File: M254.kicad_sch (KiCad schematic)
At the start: 14 parts, among them J1 from Sensor, J2 to M304, U1 NJM2903

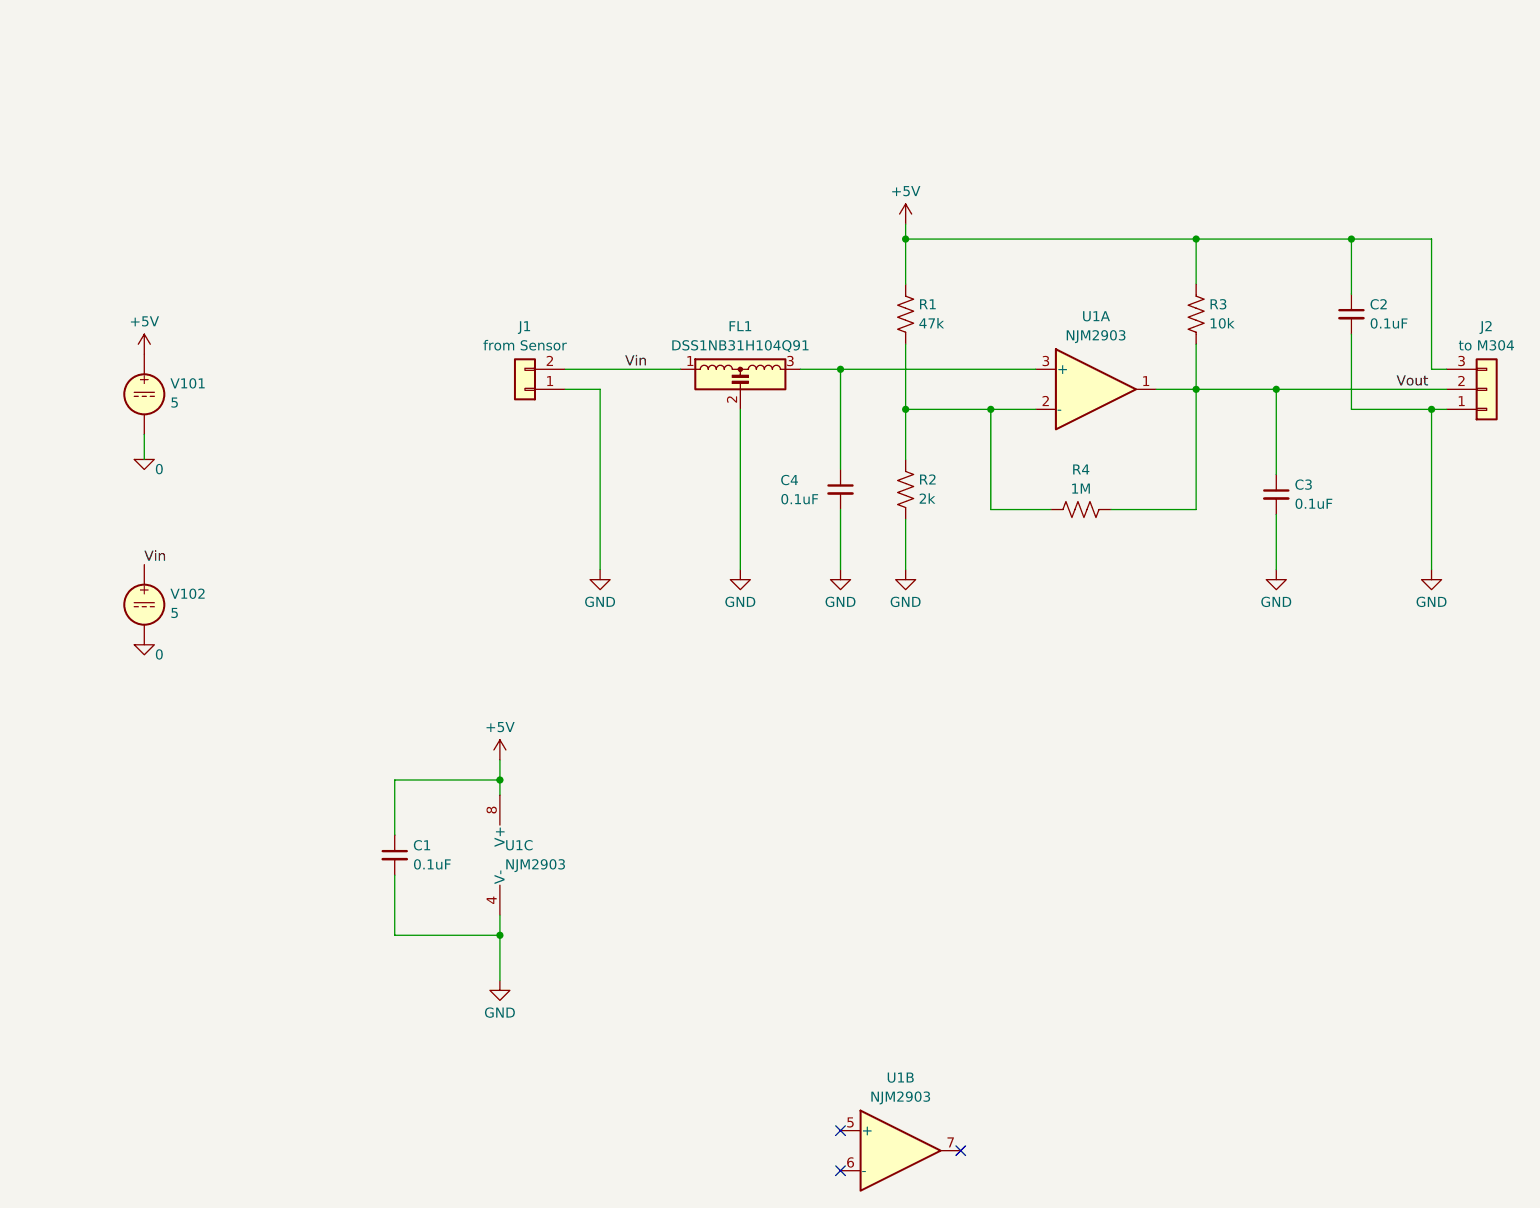
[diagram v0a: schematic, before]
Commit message: 途中
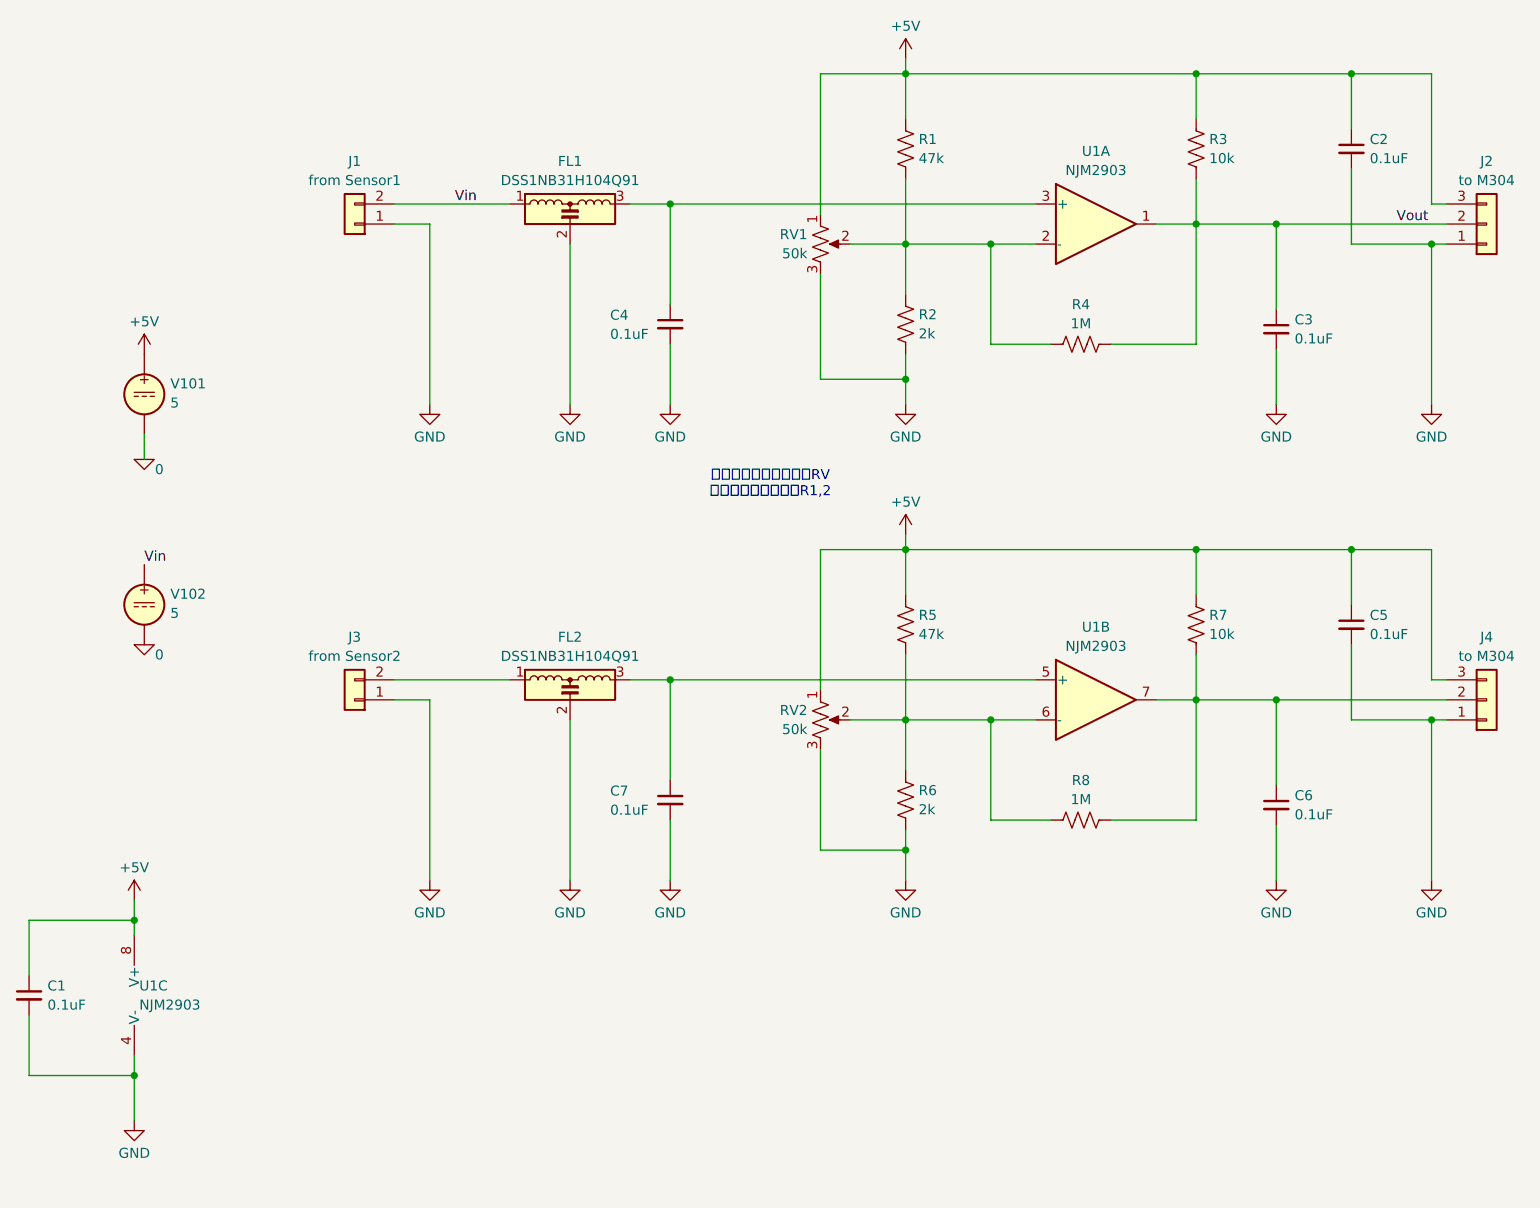
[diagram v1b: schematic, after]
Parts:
- added C5, C6, C7: 0.1uF, Capacitor_THT:C_Disc_D3.4mm_W2.1mm_P2.50mm, symbol Device:C_Small
- added FL2: DSS1NB31H104Q91, HOLLY2:DSS1, symbol Device:Filter_EMI_LCL
- added J3: from Sensor2, Connector_JST:JST_XH_B2B-XH-A_1x02_P2.50mm_Vertical, symbol Connector_Generic:Conn_01x02
- added J4: to M304, Connector_JST:JST_XH_B3B-XH-A_1x03_P2.50mm_Vertical, symbol Connector_Generic:Conn_01x03
- added R5: 47k, Resistor_THT:R_Axial_DIN0207_L6.3mm_D2.5mm_P2.54mm_Vertical, symbol Device:R_US
- added R6: 2k, Resistor_THT:R_Axial_DIN0207_L6.3mm_D2.5mm_P2.54mm_Vertical, symbol Device:R_US
- added R7: 10k, Resistor_THT:R_Axial_DIN0207_L6.3mm_D2.5mm_P2.54mm_Vertical, symbol Device:R_US
- added R8: 1M, Resistor_THT:R_Axial_DIN0207_L6.3mm_D2.5mm_P2.54mm_Vertical, symbol Device:R_US
- added RV1, RV2: 50k, Potentiometer_THT:Potentiometer_Bourns_3296W_Vertical, symbol Device:R_Potentiometer_US
- FL1: footprint holly:DSS1 -> HOLLY2:DSS1
- J1: value from Sensor -> from Sensor1
- R1, R2, R3, R4: footprint Resistor_THT:R_Axial_DIN0207_L6.3mm_D2.5mm_P10.16mm_Horizontal -> Resistor_THT:R_Axial_DIN0207_L6.3mm_D2.5mm_P2.54mm_Vertical
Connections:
- net +5V: now also C5.1, J4.3 (Pin_3), R5.1, R7.1, RV1.1, RV2.1
- net GND: now also C5.2, C6.2, C7.2, FL2.2, J3.1 (Pin_1), J4.1 (Pin_1), R6.2, RV1.3, RV2.3
- net at R1.2, R2.1, R4.1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: now also RV1.2
- net at U1.5 (+): now also C7.1, FL2.3
- net at U1.6 (-): now also R5.2, R6.1, R8.1, RV2.2
- net at U1.7: now also C6.1, J4.2 (Pin_2), R7.2, R8.2
- new net: FL2.1, J3.2 (Pin_2)
- no-connect marks 3 -> 0
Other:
- note added: "可変させたいときにはRV 固定させるときにはR1,2"
- moved on the sheet: C1, C2, C3, C4, FL1, J1, J2, R1, R2, R3, R4, U1A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
